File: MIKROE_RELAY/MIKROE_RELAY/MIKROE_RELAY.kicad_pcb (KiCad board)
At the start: 2 copper layers, 37.8 x 53.7 mm, 24 parts, among them J1 RELAY1, J2 RELAY2, J3 Screw_Terminal_01x04, K1 SRD-05VDC-SL-C, K2 SRD-05VDC-SL-C, Q1 Q_NMOS_Depletion_GSD, Q2 Q_NMOS_Depletion_GSD, U2 B0505S-2WR3, U3 PC817, U4 PC817

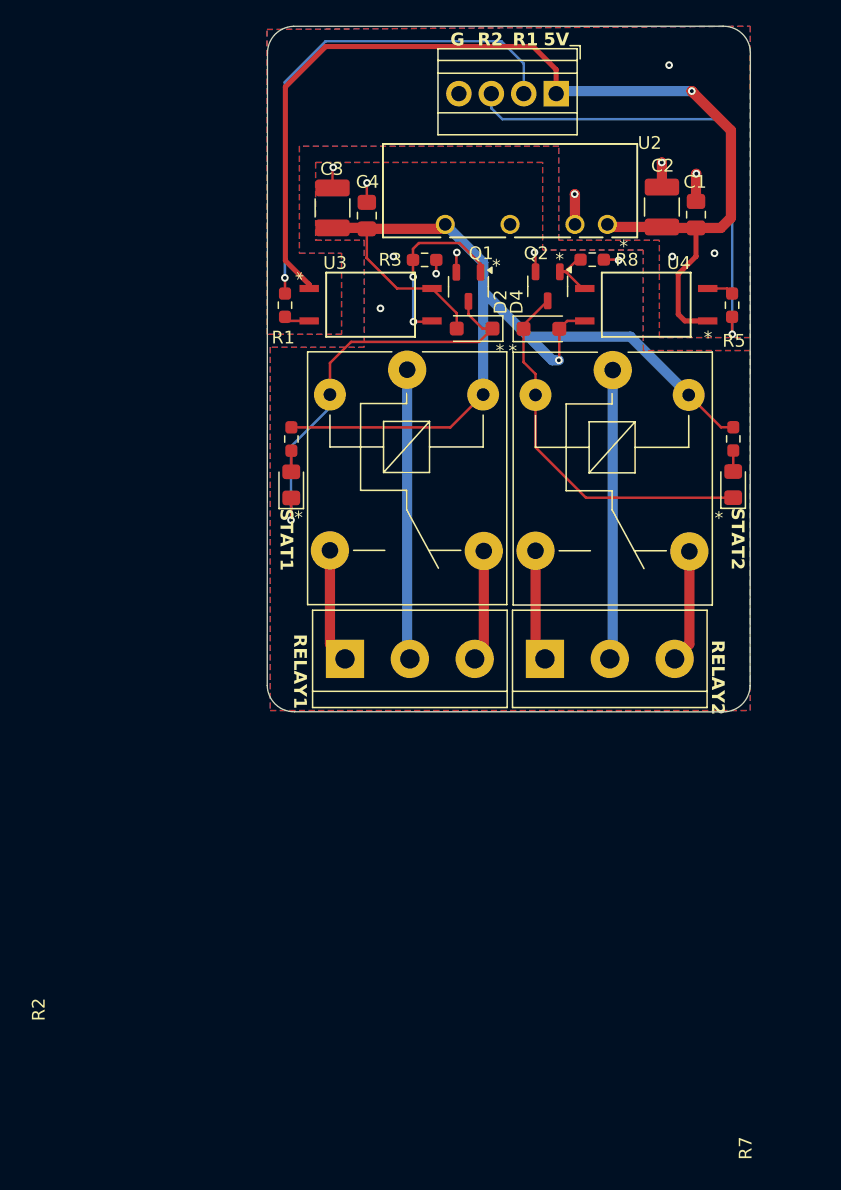
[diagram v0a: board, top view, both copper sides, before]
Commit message: -
updated silk
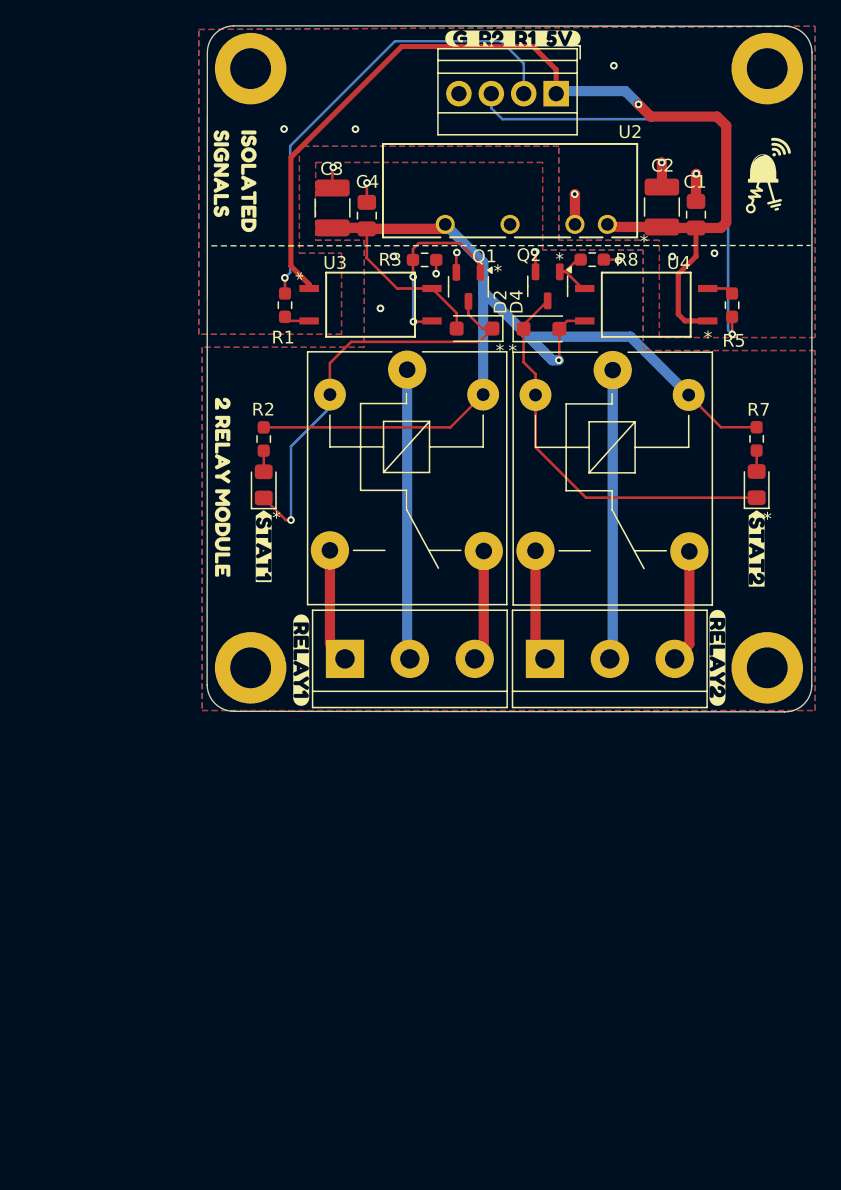
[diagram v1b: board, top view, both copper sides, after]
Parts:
- added G***: LOGO, logo:logo2, F.Cu at (139.5, 48.1)
- added H1: MountingHole, MountingHole:MountingHole_3.2mm_M3_DIN965_Pad, F.Cu at (104.6, 40.1)
- added H2: MountingHole, MountingHole:MountingHole_3.2mm_M3_DIN965_Pad, F.Cu at (145.1, 40.1)
- added H3: MountingHole, MountingHole:MountingHole_3.2mm_M3_DIN965_Pad, F.Cu at (104.6, 87.1)
- added H4: MountingHole, MountingHole:MountingHole_3.2mm_M3_DIN965_Pad, F.Cu at (145.1, 87.1)
- added kibuzzard-6720ECCE: G***, kibuzzard-6720ECCE, F.Cu at (105.7, 77.5)
- added kibuzzard-6720ECE8: G***, kibuzzard-6720ECE8, F.Cu at (144.3, 77.7)
- added kibuzzard-6720EF98: G***, kibuzzard-6720EF98, F.Cu at (125.2, 37.8)
- added kibuzzard-6720F047: G***, kibuzzard-6720F047, B.Cu at (125.2, 37.8)
- added kibuzzard-6720F077: G***, kibuzzard-6720F077, F.Cu at (141.2, 86.3)
- added kibuzzard-6720F077: G***, kibuzzard-6720F077, B.Cu at (141.2, 86.3)
- added kibuzzard-6720F294: G***, kibuzzard-6720F294, F.Cu at (108.6, 86.5)
- added kibuzzard-6720F294: G***, kibuzzard-6720F294, B.Cu at (108.5, 86.5)
- added kibuzzard-6720F424: G***, kibuzzard-6720F424, B.Cu at (112.1, 89.4)
- added kibuzzard-6720F448: G***, kibuzzard-6720F448, B.Cu at (122.3, 89.4)
- added kibuzzard-6720F477: G***, kibuzzard-6720F477, B.Cu at (127.5, 89.4)
- added kibuzzard-6720F484: G***, kibuzzard-6720F484, B.Cu at (138.2, 89.4)
- added kibuzzard-6720F4CB: G***, kibuzzard-6720F4CB, B.Cu at (117.2, 89.4)
- added kibuzzard-6720F4E3: G***, kibuzzard-6720F4E3, B.Cu at (132.9, 89.4)
- added kibuzzard-6720F54C: G***, kibuzzard-6720F54C, F.Cu at (102.5, 72.9)
- added kibuzzard-6720F708: G***, kibuzzard-6720F708, F.Cu at (103.4, 49.0)
- moved R2 2.17 mm to (105.7, 69.2)
- moved D1 2.16 mm to (105.7, 72.8)
- moved D3 1.84 mm to (144.3, 72.7)
- moved R7 1.83 mm to (144.3, 69.2)
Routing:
- net 5V_ISO: track 83.9 -> 79.4 mm
- net 5V_RLY: track 86.2 -> 90.2 mm
- net /RE1: track 39.7 -> 36.5 mm
- net Net-(D3-K): track 29.8 -> 31.6 mm
- net Net-(D1-K): track 32.5 -> 33.6 mm
- net GNDD: vias 6 -> 8
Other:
- board size 37.8 x 53.7 mm -> 47.4 x 53.7 mm
- board text removed: "5V"
- board text removed: "COM1"
- board text removed: "COM2"
- board text removed: "G"
- board text removed: "NC1"
- board text removed: "NC2"
- board text removed: "NO1"
- board text removed: "NO2"
- board text removed: "R1"
- board text removed: "R2"
- board text removed: "RELAY1"
- board text removed: "RELAY2"
- board text removed: "STAT1"
- board text removed: "STAT2"
